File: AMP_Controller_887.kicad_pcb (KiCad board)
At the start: 2 copper layers, 79 x 61.5 mm, 65 parts, among them J1 Conn_PIC_ICSP_ICD, J3 4P_I2C, J4 Conn_01x13_Socket, J5 Conn_01x13_Socket, J6 2P_POWER, J7 USB_Mini_B_90_Angled, SW1 SW_RST, SW2 SW_PR21, X1 16MHz

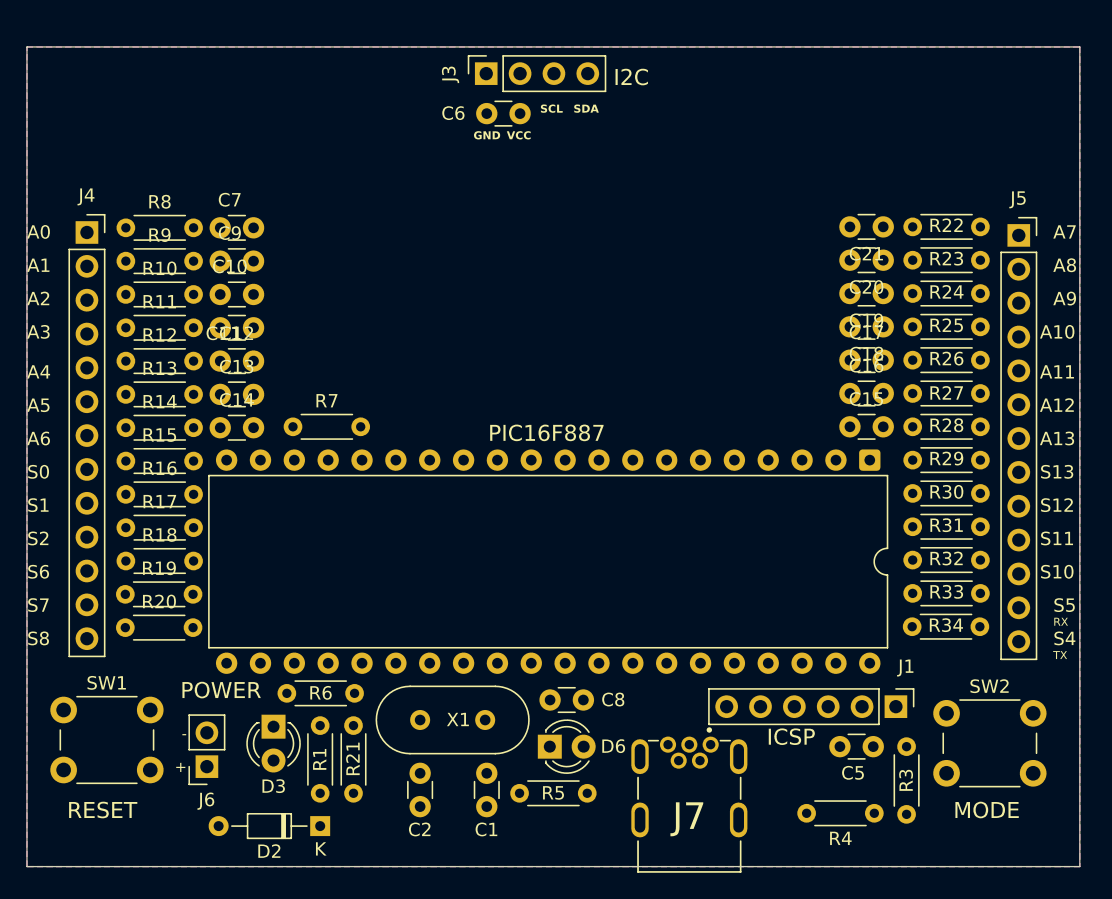
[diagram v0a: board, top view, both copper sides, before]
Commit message: Finished layout.
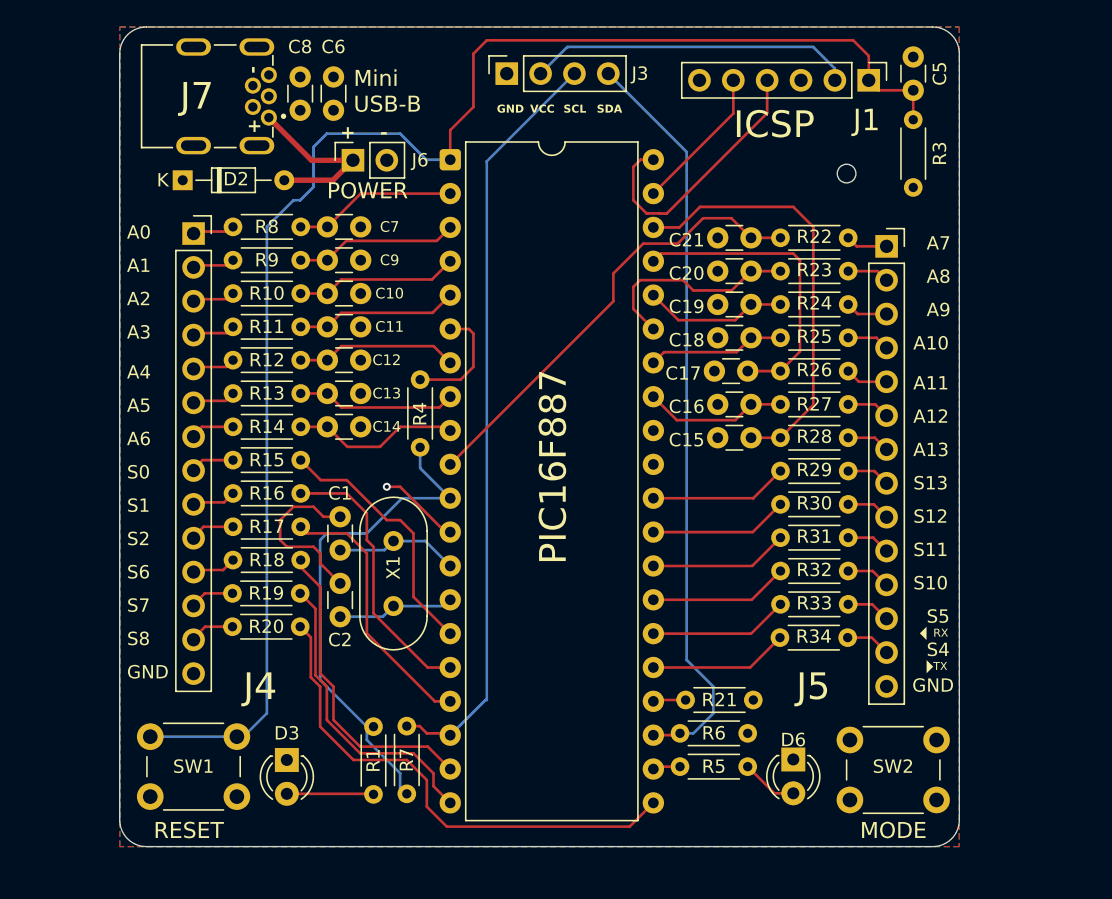
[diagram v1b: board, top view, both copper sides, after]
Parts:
- J4, J5: footprint Connector_PinSocket_2.54mm:PinSocket_1x13_P2.54mm_Vertical -> Connector_PinSocket_2.54mm:PinSocket_1x14_P2.54mm_Vertical
- moved J7 59.2 mm to (76.8, 36.7), turned to 90 degrees
- moved C5 52.0 mm to (126.0, 33.8), turned to -90 degrees
- moved D2 49.5 mm to (71.2, 43.0), turned to 0 degrees
- moved C8 49.1 mm to (80.0, 37.8), turned to 90 degrees
- moved J1 47.0 mm to (122.7, 35.5)
- moved R3 47.0 mm to (126.0, 43.5)
- moved J6 46.8 mm to (84.0, 41.5), turned to 90 degrees
- moved R4 43.8 mm to (89.0, 63.0), turned to 90 degrees
- moved PIC16F887 38.7 mm to (91.3, 41.5), turned to 0 degrees
- moved R6 29.7 mm to (108.5, 84.5)
- moved R21 25.0 mm to (108.9, 82.0), turned to 0 degrees
- moved R7 24.0 mm to (88.0, 84.0), turned to -90 degrees
- moved C1 20.0 mm to (83.0, 70.8), turned to 90 degrees
- moved D6 18.3 mm to (117.0, 86.5), turned to -90 degrees
- moved C2 13.2 mm to (83.0, 75.8), turned to 90 degrees
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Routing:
- net /MCLR: track 0.00 -> 112.6 mm
- net VCC: track 0.00 -> 61.8 mm
- net /SCL: track 0.00 -> 57.2 mm
- net /SDA: track 0.00 -> 56.4 mm
- net /SW8: track 0.00 -> 38.1 mm
- net /AN7: track 0.00 -> 34.3 mm
- net /AN13: track 0.00 -> 32.3 mm
- net /SW6: track 0.00 -> 23.4 mm
- net /AN11: track 0.00 -> 22.8 mm
- net /SW7: track 0.00 -> 22.7 mm
- net /SW1: track 0.00 -> 20.7 mm
- net /PGD: track 0.00 -> 20.3 mm
- net /SW2: track 0.00 -> 20.2 mm
- net /SW0: track 0.00 -> 19.4 mm
- net GND: track 0.00 -> 19.2 mm, vias 0 -> 1
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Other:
- board size 79 x 61.5 mm -> 63 x 61.5 mm
- board text added: "11mm"
- board text added: "8.5mm"
- board text added: "AMP_Controller_PIC16F887 Rev.1 17th, April 2025 Made by @deulamco"
- board text added: "KiCAD"
- board text added: "Made with"
- board text added: "Mini USB-B"
- board text removed: "I2C"
